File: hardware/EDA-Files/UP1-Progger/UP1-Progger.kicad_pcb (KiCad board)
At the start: 2 copper layers, 29.2 x 33.7 mm, 12 parts, among them J1 UP1_Prog_Connector, J11 UP1_Prog_Connector, J2 USB_B_Micro, J4 SWD_Interface, J5 ST Link V2 Clone, SW1 Reset, SW2 Bootsel, U1 LDO_3V3_SOT23-3

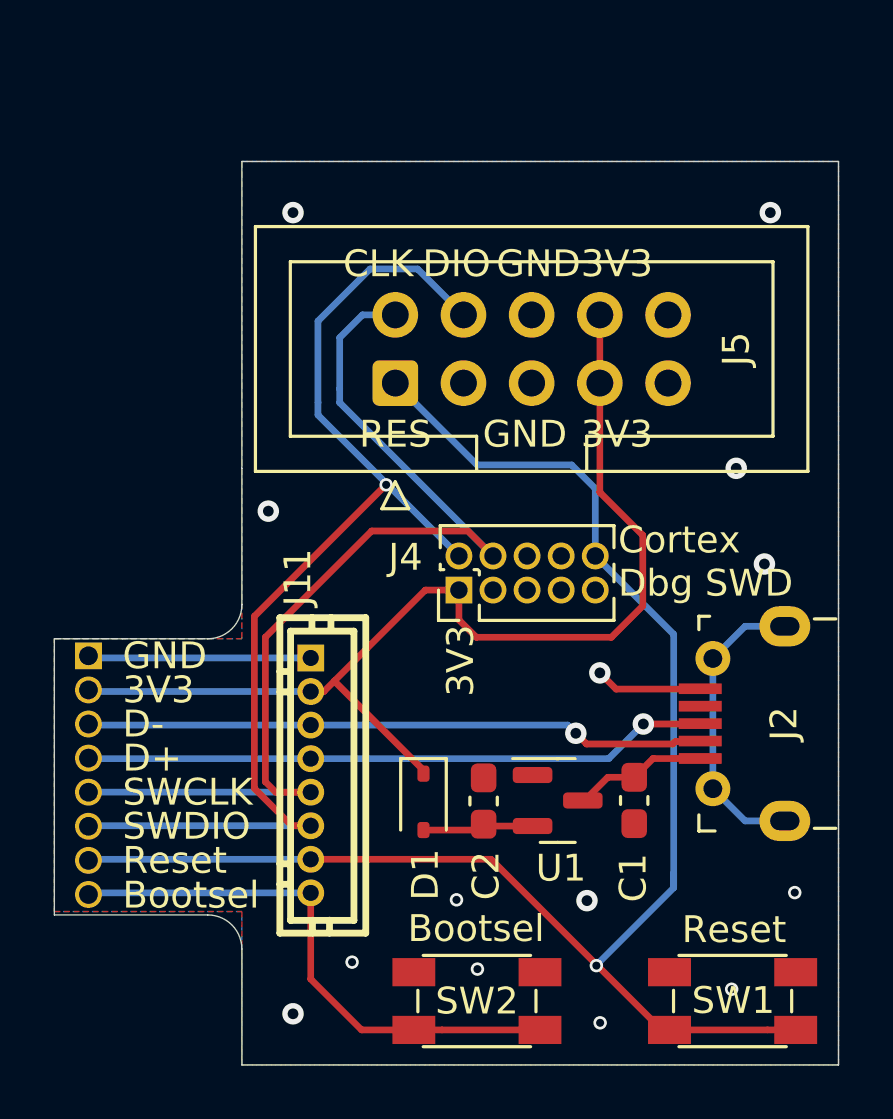
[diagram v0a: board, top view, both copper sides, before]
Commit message: wip progger
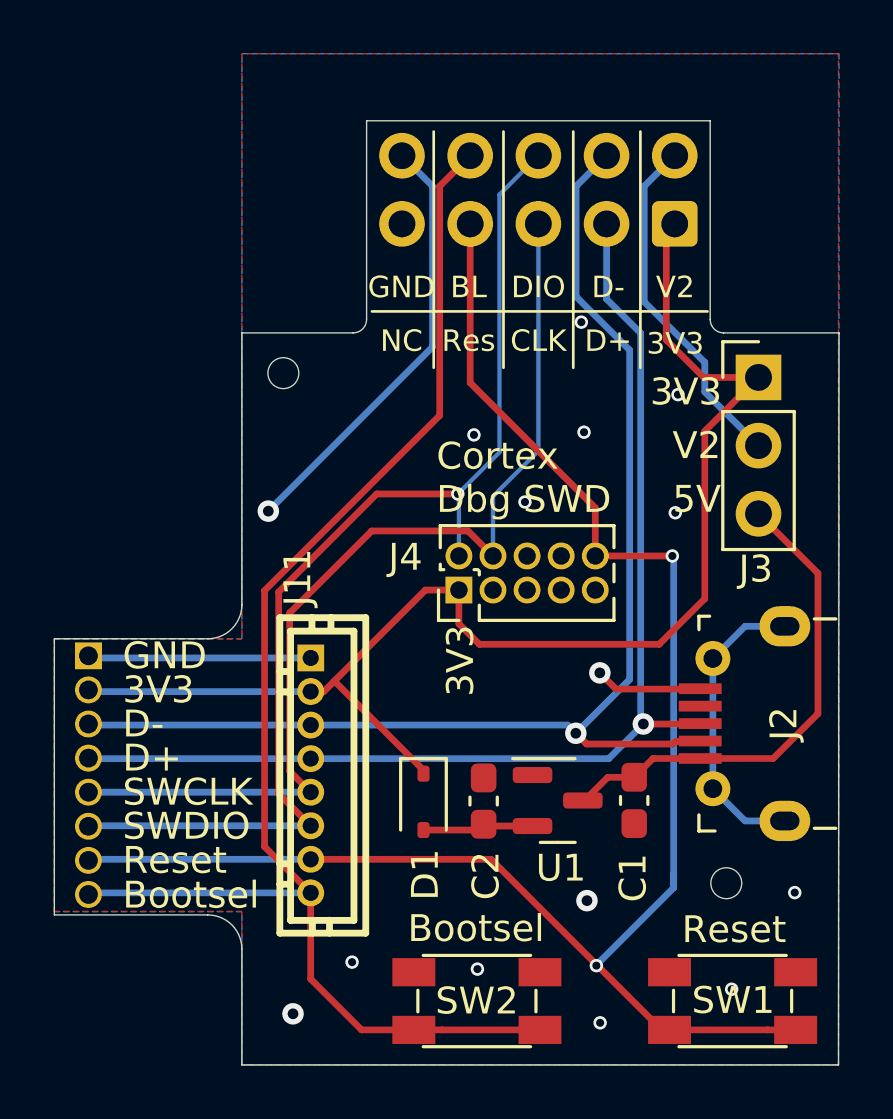
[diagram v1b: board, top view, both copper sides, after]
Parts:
- removed the G*** at (103.5, 116.8)
- added G***: LOGO, OpenKNX:OpenKNX_Logo_10x10, B.Cu at (113.0, 106.1)
- added G***: LOGO, OpenKNX:CC-BY-NY-SA_12x4, B.Cu at (103.9, 104.3)
- added J3: Conn_01x03, Connector_PinHeader_2.54mm:PinHeader_1x03_P2.54mm_Vertical, F.Cu at (116.4, 102.7)
- added REF**: JLCPCB_Tooling_hole, DomsKiCADLib:JLCPCB_Tooling_hole, F.Cu at (115.2, 121.5)
- added REF**: JLCPCB_Tooling_hole, DomsKiCADLib:JLCPCB_Tooling_hole, F.Cu at (98.7, 102.5)
- J5: moved to B.Cu
- moved J5 12.0 mm to (113.3, 96.9)
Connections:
- J5 pad 1: Reset -> +3.3V
- J5 pad 10: unconnected-(J5-Pin_10-Pad10) -> GND
- J5 pad 2: SWCLK -> Net-(J3-Pin_2)
- J5 pad 3: unconnected-(J5-Pin_3-Pad3) -> D+
- J5 pad 4: SWDIO -> D-
- J5 pad 5: GND -> SWCLK
- J5 pad 6: GND -> SWDIO
- J5 pad 7: +3.3V -> Reset
- J5 pad 8: +3.3V -> Bootsel
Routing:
- net Bootsel: track 20.8 -> 52.2 mm
- net D-: track 23.1 -> 46.8 mm
- net D+: track 23.3 -> 42.5 mm
- net GND: track 12.3 -> 28.5 mm, vias 14 -> 15
- net +5V: track 4.96 -> 18.4 mm
- net Net-(J3-Pin_2): track 0.00 -> 13.0 mm
- net +3.3V: track 40.4 -> 49.2 mm
- net Reset: track 58.7 -> 63.1 mm, vias 1 -> 2
- net SWCLK: track 38.9 -> 37.6 mm
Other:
- board size 29.2 x 33.7 mm -> 29.2 x 35.2 mm
- board text added: "5V"
- board text added: "BL"
- board text added: "NC"
- board text added: "Res"
- board text added: "UP1-Progger V01.10 by Ing-Dom, 2024"
- board text added: "V2"
- board text removed: "Ing-Dom, 2023"
- board text removed: "RES"
- board text removed: "UP1-Progger"
- board text removed: "V01.00"
